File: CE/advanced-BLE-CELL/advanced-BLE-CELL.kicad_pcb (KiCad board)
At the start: 4 copper layers, 65 x 56 mm, 24 parts, among them J3 40HAT, J6 CONN_02X02, J9 CONN_01X02, Q1 DMG2305UX, Q2 DMMT5401, U1 nRF52840, U2 CAT24C32, U3 BG96

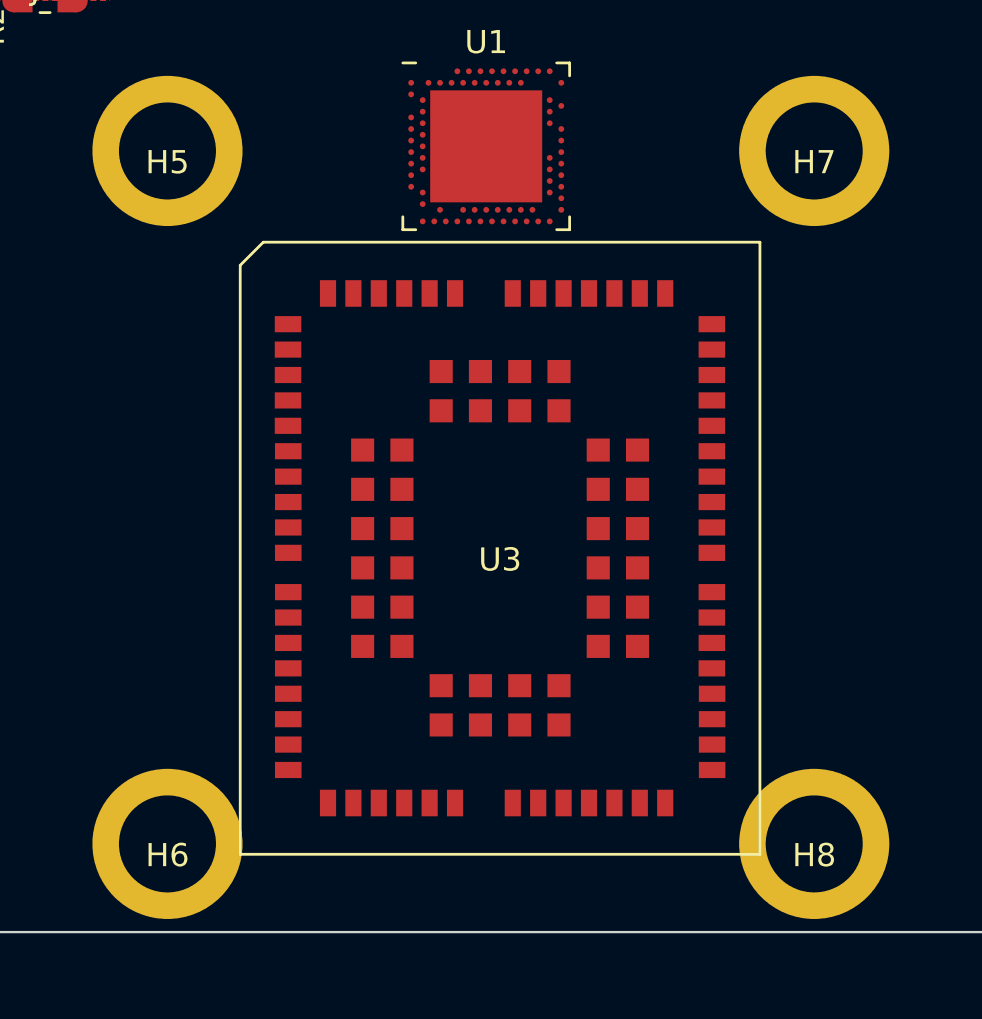
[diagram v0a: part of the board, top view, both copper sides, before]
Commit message: asdf
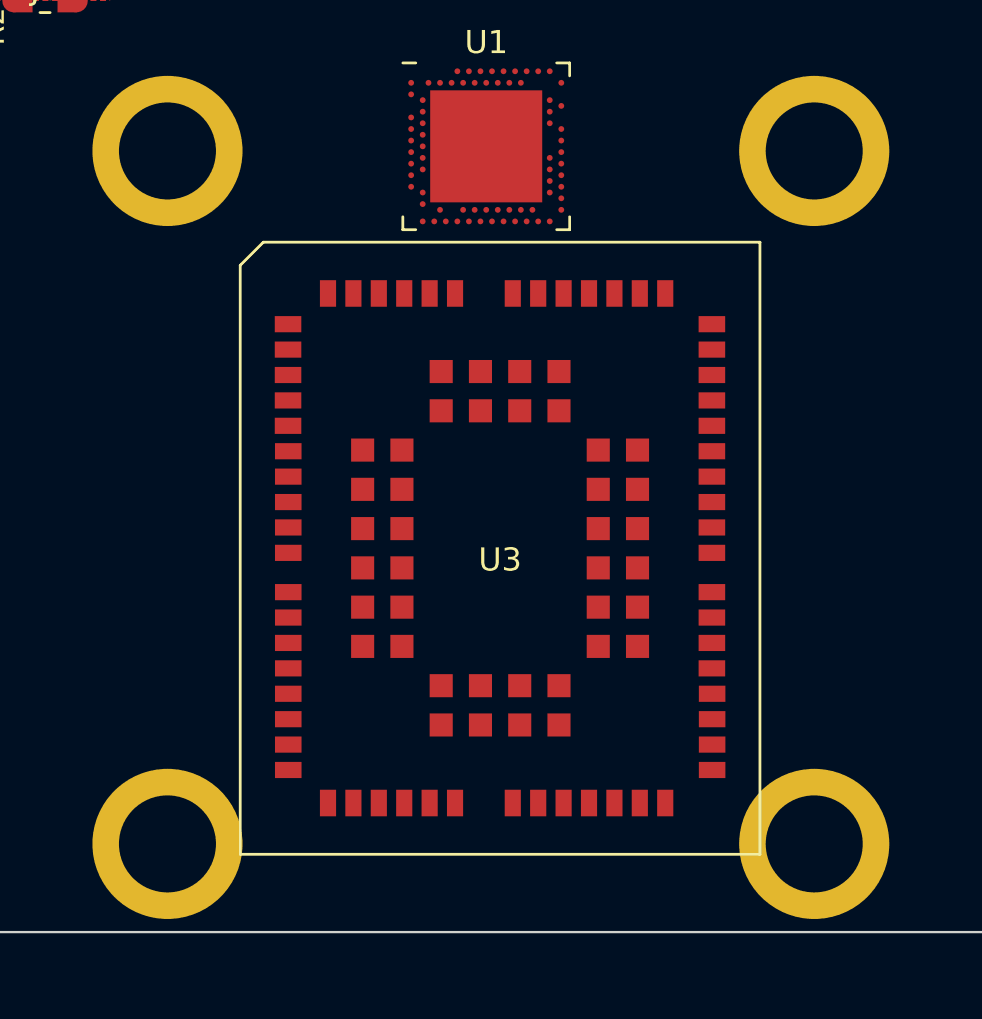
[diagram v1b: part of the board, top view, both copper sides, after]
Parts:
- H5, H6, H7, H8: footprint ABC:4881 -> ABC:4881-Top; moved to B.Cu
